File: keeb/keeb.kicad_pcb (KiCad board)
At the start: 2 copper layers, 138 parts, among them J1 USB_A, J2 USB_A, J3 USB_A, J4 USB_A, P1 USB_C_Plug_USB2.0, P2 USB_C_Plug_USB2.0, SW1 SW_Push, SW10 SW_Push, SW11 SW_Push, SW12 SW_Push, SW13 SW_Push, SW14 SW_Push, SW15 SW_Push, SW16 SW_Push, SW17 SW_Push, SW18 SW_Push, SW19 SW_Push, SW2 SW_Push, SW20 SW_Push, SW21 SW_Push, SW22 SW_Push, SW23 SW_Push, SW24 SW_Push, SW25 SW_Push, SW26 SW_Push, SW27 SW_Push, SW28 SW_Push, SW29 SW_Push, SW3 SW_Push, SW30 SW_Push, SW31 SW_Push, SW32 SW_Push, SW33 SW_Push, SW34 SW_Push, SW35 SW_Push, SW36 SW_Push, SW37 SW_Push, SW38 SW_Push, SW39 SW_Push, SW4 SW_Push, SW40 SW_Push, SW41 SW_Push, SW42 SW_Push, SW43 SW_Push, SW44 SW_Push, SW45 SW_Push, SW46 SW_Push, SW47 SW_Push, SW48 SW_Push, SW49 SW_Push, SW5 SW_Push, SW50 SW_Push, SW6 SW_Push, SW7 SW_Push, SW8 SW_Push, SW9 SW_Push, U1 XIAO-nRF52840-SMD, U2 XIAO-nRF52840-SMD, U3 USB2512-AEZG, U4 USB2512-AEZG

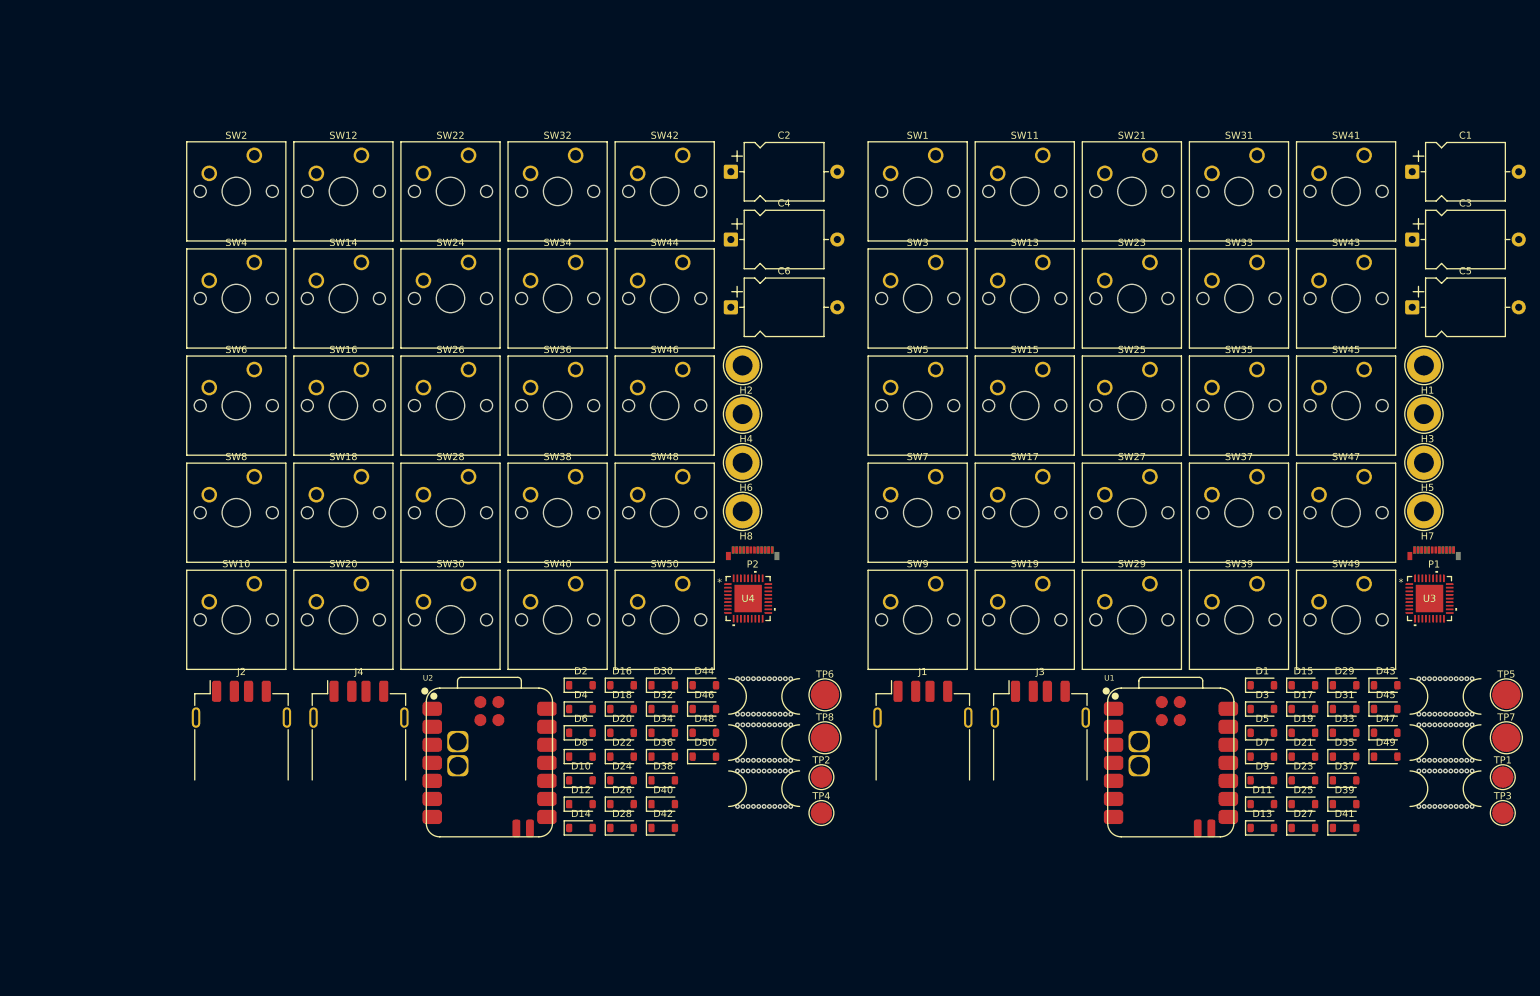
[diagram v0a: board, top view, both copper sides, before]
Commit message: worked on routing
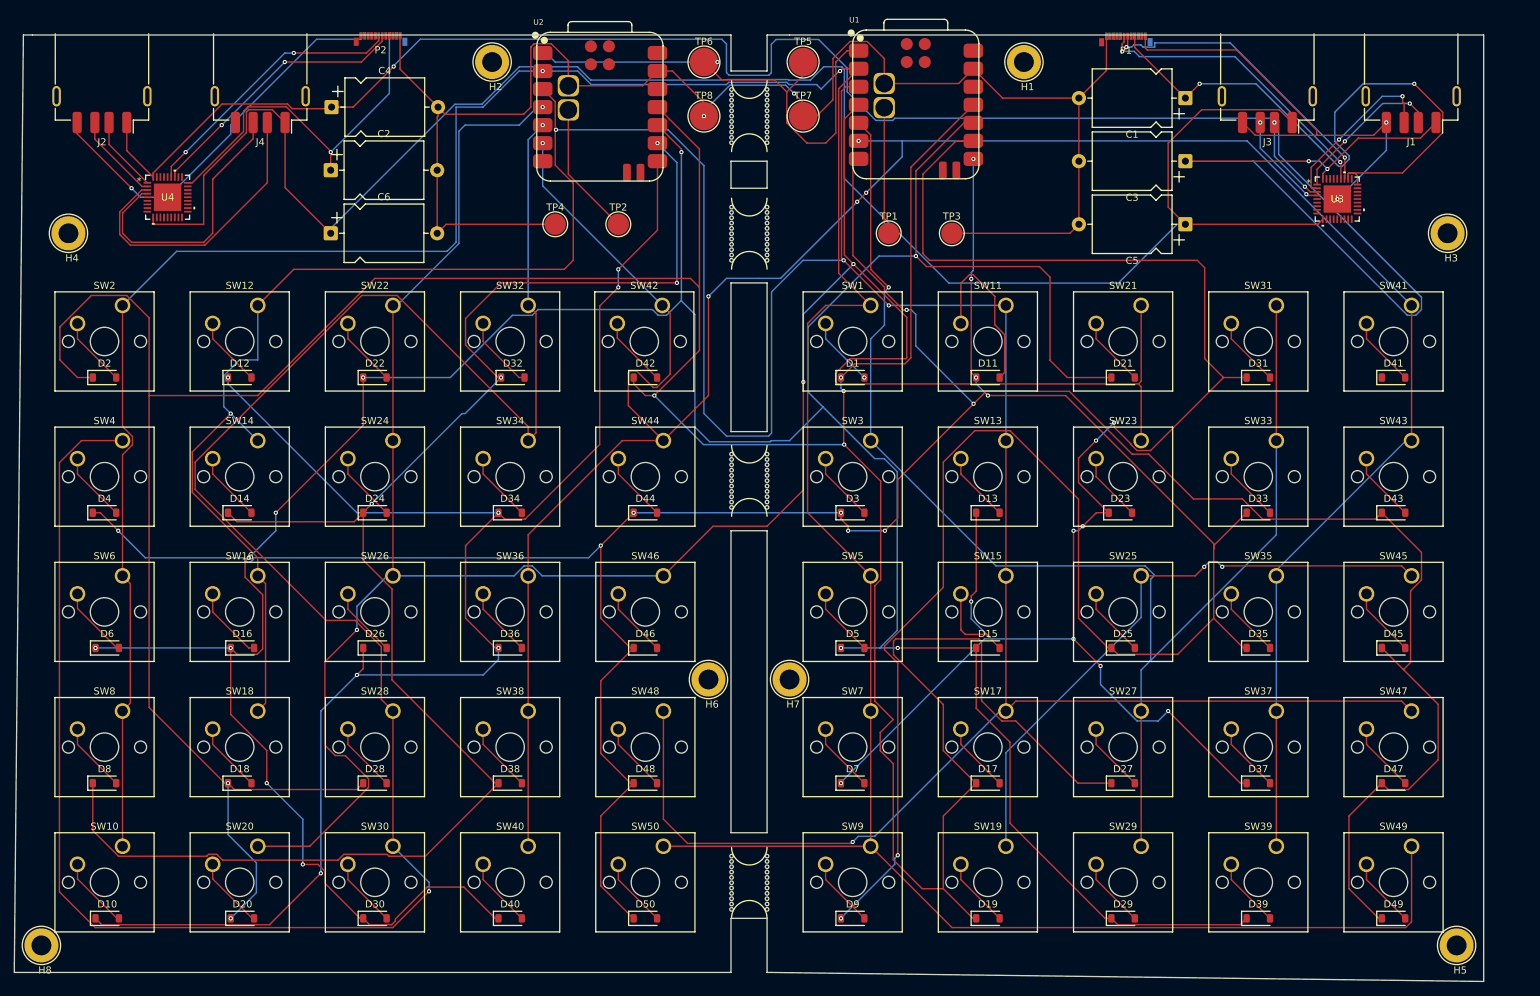
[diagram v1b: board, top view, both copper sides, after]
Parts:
- removed H11, H13: MountingHole, keeb:mouse-bite-5mm-slot
- TP5, TP6: value HapticFeedbackMotor+ -> Motor+
- TP7, TP8: value HapticFeedbackMotor- -> Motor-
- moved TP5 133.3 mm to (146.7, 33.0)
- moved TP7 132.2 mm to (146.7, 40.6)
- moved J1 117.0 mm to (232.4, 34.3), turned to 180 degrees
- moved H8 116.2 mm to (39.4, 157.5)
- moved TP1 115.6 mm to (158.8, 57.1)
- moved TP3 112.7 mm to (167.6, 57.1)
- moved H9 102.7 mm to (139.1, 92.0), turned to 90 degrees
- moved J3 99.9 mm to (212.1, 34.3), turned to 180 degrees
- moved U1 99.4 mm to (162.6, 39.0)
- moved U4 99.4 mm to (57.1, 52.1)
- moved H4 98.3 mm to (43.2, 57.1)
- moved J2 96.7 mm to (47.9, 34.3), turned to 180 degrees
- moved J4 95.7 mm to (70.2, 34.3), turned to 180 degrees
- moved U2 93.7 mm to (118.1, 39.4)
- moved H7 92.5 mm to (144.8, 120.0)
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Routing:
- net row0: track 0.00 -> 527.5 mm, vias 0 -> 6
- net col3: track 0.00 -> 507.8 mm, vias 0 -> 3
- net col1: track 0.00 -> 487.3 mm, vias 0 -> 5
- net row1: track 0.00 -> 478.3 mm, vias 0 -> 11
- net row2: track 0.00 -> 464.0 mm, vias 0 -> 13
- net row3: track 0.00 -> 459.3 mm, vias 0 -> 13
- net col0: track 0.00 -> 454.1 mm, vias 0 -> 2
- net col2: track 0.00 -> 435.7 mm, vias 0 -> 6
- net row4: track 0.00 -> 391.6 mm, vias 0 -> 8
- net col4: track 0.00 -> 360.4 mm, vias 0 -> 5
- net GND: track 0.00 -> 341.8 mm, vias 0 -> 5
- net downVbus0: track 0.00 -> 310.5 mm, vias 0 -> 3
- net downVbus1: track 0.00 -> 260.3 mm
- net Net-(U3-VBUS_DET): track 0.00 -> 88.4 mm, vias 0 -> 2
- net data0: track 0.00 -> 70.9 mm, vias 0 -> 1
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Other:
- board outline added: 207 x 133.3 mm
